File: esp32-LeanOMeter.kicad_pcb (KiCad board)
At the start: 2 copper layers, 90 x 66 mm, 4 parts, among them J1 Conn_01x06-SdCard, J2 Conn_02x15_Counter_Clockwise, J3 Conn_01x04-GpsModuleNeoM8N, J4 Conn_01x10-BNO085

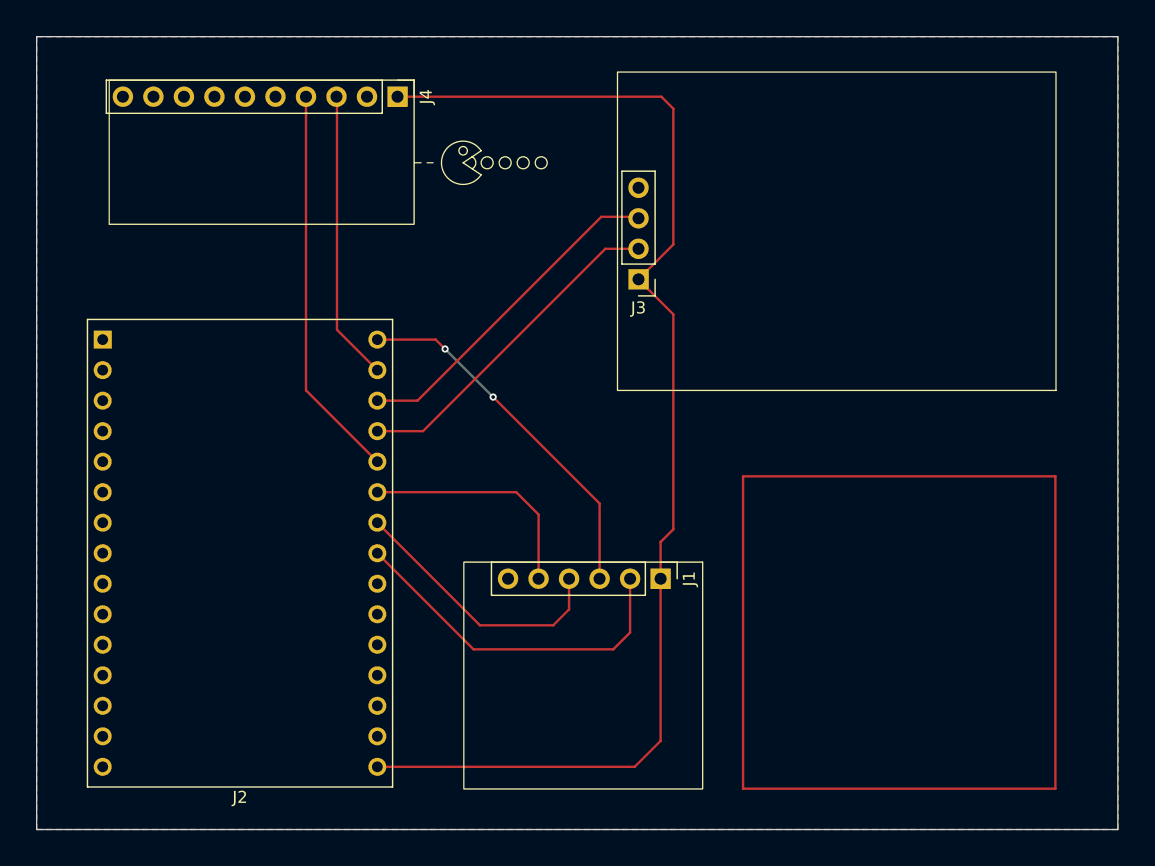
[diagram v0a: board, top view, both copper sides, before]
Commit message: changed a few things. need drill holes
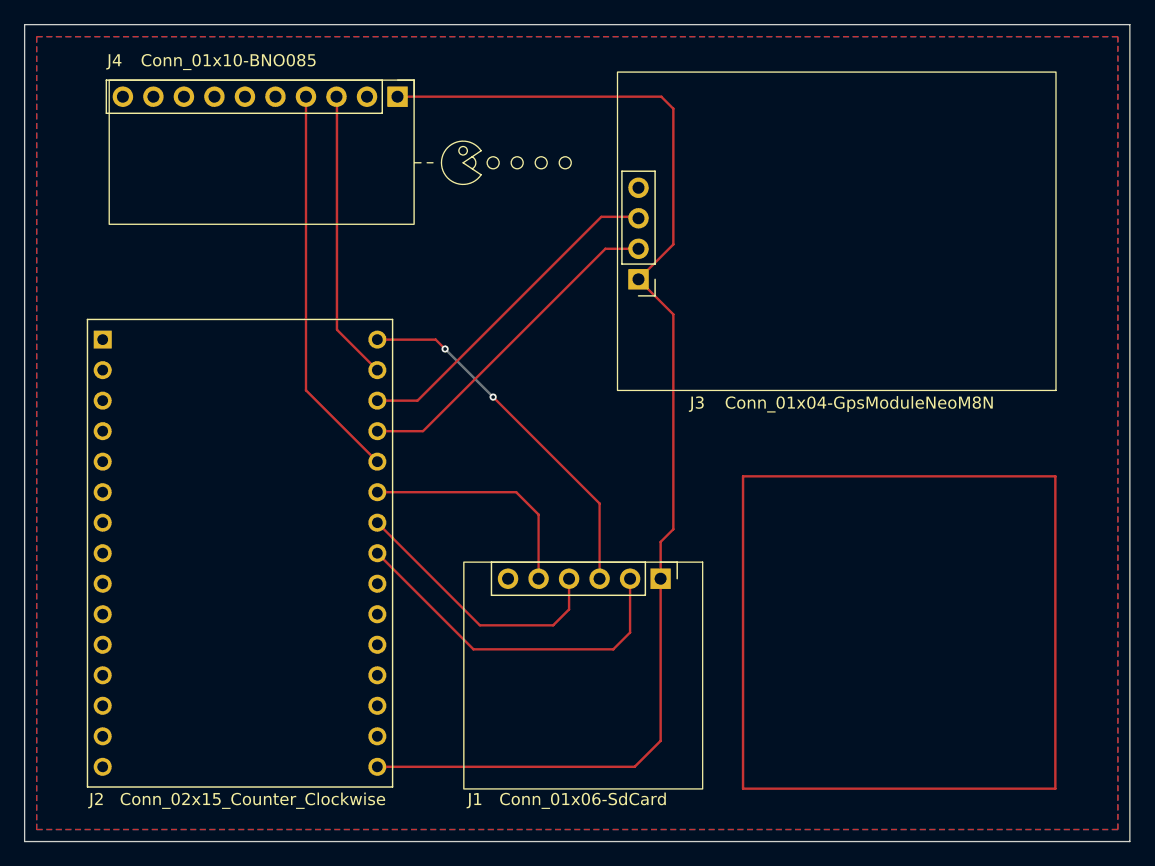
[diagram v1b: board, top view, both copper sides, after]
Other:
- board size 90 x 66 mm -> 92 x 68 mm
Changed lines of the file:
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@@
 		(tags "Through hole pin header THT 1x10 2.54mm single row")
 		(property "Reference" "J4"
-			(at 0 -2.38 90)
+			(at -3 23.54 180)
 			(layer "F.SilkS")
 			(effects
@@
 		)
 		(property "Value" "Conn_01x10-BNO085"
-			(at -3 16.04 180)
-			(layer "F.Fab")
+			(at -3 14.04 180)
+			(layer "F.SilkS")
 			(effects
 				(font
@@
 		(tags "Through hole pin header THT 1x06 2.54mm single row")
 		(property "Reference" "J1"
-			(at 0 -2.38 90)
+			(at 18.3775 15.44 180)
 			(layer "F.SilkS")
 			(effects
@@
 		)
 		(property "Value" "Conn_01x06-SdCard"
-			(at -3.1225 8.94 180)
-			(layer "F.Fab")
+			(at 18.3775 6.44 180)
+			(layer "F.SilkS")
 			(effects
 				(font
@@
 		(tags "Through hole pin header THT 1x04 2.54mm single row")
 		(property "Reference" "J3"
-			(at 0 -2.38 0)
+			(at -4.9 -10.3 0)
 			(layer "F.SilkS")
 			(effects
@@
 		)
 		(property "Value" "Conn_01x04-GpsModuleNeoM8N"
-			(at -9.9 -9.8 0)
-			(layer "F.Fab")
+			(at -18.4 -10.3 0)
+			(layer "F.SilkS")
 			(effects
 				(font
@@
 		(tags "esp32 esp32-c3 riscv risc-v wifi bluetooth ble")
 		(property "Reference" "J2"
-			(at 11.43 38.1 0)
+			(at -0.5 38.28 0)
 			(unlocked yes)
 			(layer "F.SilkS")
@@
 		)
 		(property "Value" "Conn_02x15_Counter_Clockwise"
-			(at 11.43 40.64 0)
+			(at 12.5 38.28 0)
 			(unlocked yes)
-			(layer "F.Fab")
+			(layer "F.SilkS")
 			(effects
 				(font
@@
 	)
 	(gr_circle
-		(center 98.5 48.5)
-		(end 99 48.5)
+		(center 99 48.5)
+		(end 99.5 48.5)
 		(stroke
 			(width 0.1)
@@
 	)
 	(gr_circle
-		(center 100 48.5)
-		(end 100.5 48.5)
-		(stroke
-			(width 0.1)
-			(type default)
-		)
-		(fill no)
-		(layer "F.SilkS")
-	)
-	(gr_circle
-		(center 101.5 48.5)
-		(end 102 48.5)
+		(center 101 48.5)
+		(end 101.5 48.5)
 		(stroke
 			(width 0.1)
@@
 	(gr_circle
 		(center 103 48.5)
-		(end 103 49)
+		(end 103.5 48.5)
+		(stroke
+			(width 0.1)
+			(type default)
+		)
+		(fill no)
+		(layer "F.SilkS")
+	)
+	(gr_circle
+		(center 105 48.5)
+		(end 105 49)
 		(stroke
 			(width 0.1)
@@
 	)
 	(gr_rect
-		(start 61 38)
-		(end 151 104)
+		(start 60 37)
+		(end 152 105)
 		(stroke
 			(width 0.1)
